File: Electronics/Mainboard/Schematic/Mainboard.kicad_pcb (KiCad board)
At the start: 4 copper layers, 45 x 140 mm, 84 parts, among them J1 CONN_01X02, J10 CONN_01X04, J11 M1, J12 M2, J13 M3, J14 M4, J2 CONN_01X02, J3 CONN_01X02, J4 CONN_01X02, J5 CONN_01X02, J6 CONN_02X05, J7 CONN_02X10, J8 CONN_01X02, J9 CONN_01X02, Q1 BUK7Y7R8-80EX, Q2 BUK7Y7R8-80EX, Q4 BUK7Y7R8-80EX, U1 LM2678-3.3V, U10 LTC2954, U2 LM2678-12V, U4 LM5121, U6 ACS781, U7 LSM6DS33, U8 STM32F031G6U6, U9 LTC2876, Y1 Resonator_Small

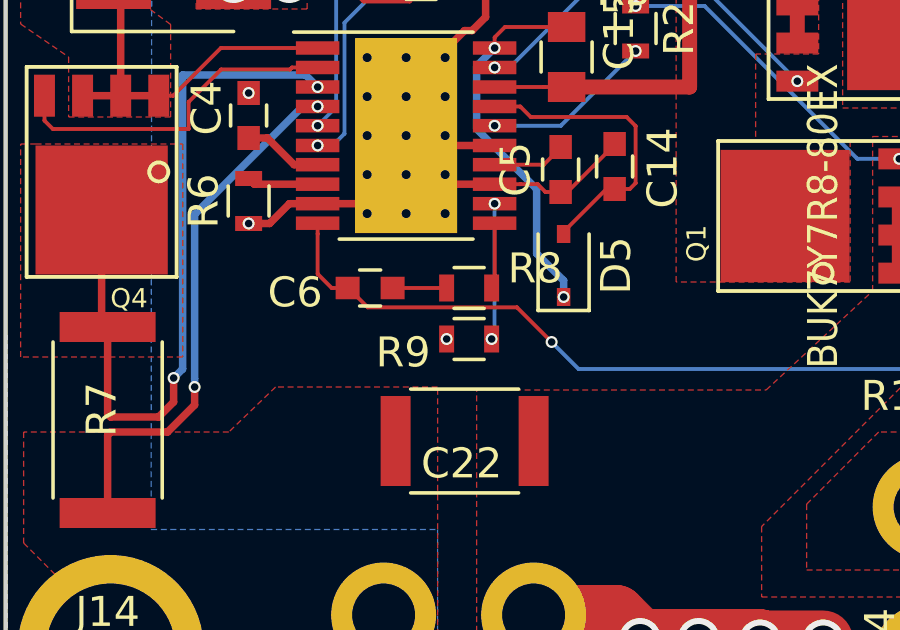
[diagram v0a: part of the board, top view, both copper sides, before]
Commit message: new mainboard
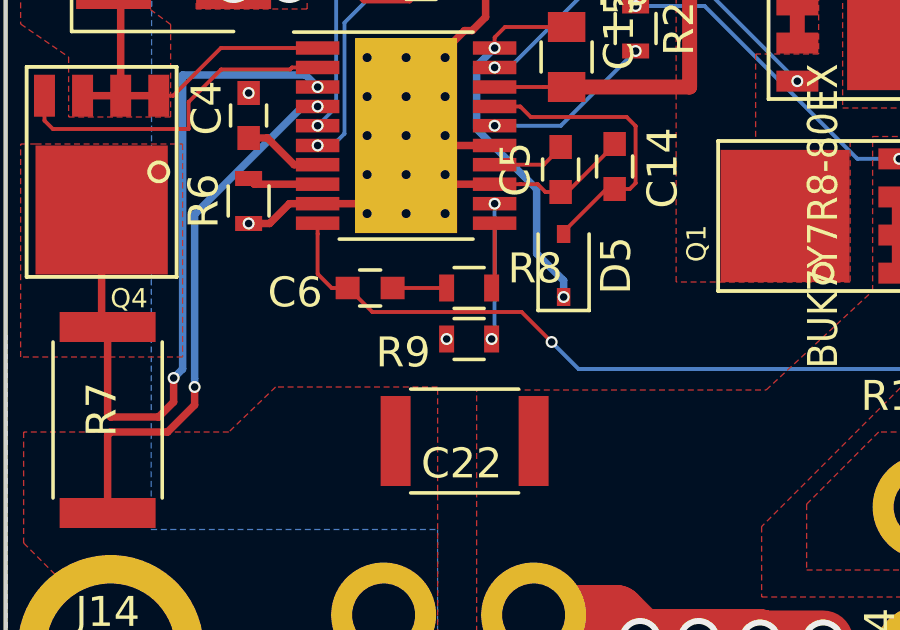
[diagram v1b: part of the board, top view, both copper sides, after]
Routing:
- net Earth: vias 56 -> 55
- net (no net): vias 0 -> 1
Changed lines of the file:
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@@
     (links 231)
     (no_connects 0)
-    (area 49.924999 29.924999 95.075001 170.075001)
+    (area 47.327142 29.924999 95.075001 170.763333)
     (thickness 1.6)
     (drawings 23)
@@
   )
   (setup
-    (last_trace_width 2)
+    (last_trace_width 0.13)
     (user_trace_width 0.13)
     (user_trace_width 0.25)
@@
     (visible_elements 7FFFEFFF)
     (pcbplotparams
-      (layerselection 0x010f0_80000001)
+      (layerselection 0x010f0_80000007)
       (usegerberextensions false)
       (excludeedgelayer true)
@@
   (gr_line (start 95 32) (end 95 168) (layer Edge.Cuts) (width 0.15))
   (gr_line (start 52 30) (end 93 30) (layer Edge.Cuts) (width 0.15))
+  (via (at 59.45 144.3) (size 1.4) (drill 1) (layers F.Cu B.Cu) (net 0))
   (via (at 54.9 99.6) (size 1.4) (drill 1) (layers F.Cu B.Cu) (net 1))
   (via (at 57.9 99.6) (size 1.4) (drill 1) (layers F.Cu B.Cu) (net 1))
-  (via (at 59.45 144.3) (size 1.4) (drill 1) (layers F.Cu B.Cu) (net 1))
   (segment (start 52.75 84.35) (end 55.35 84.35) (width 2) (layer F.Cu) (net 1))
   (via (at 55.35 84.35) (size 1.4) (drill 1) (layers F.Cu B.Cu) (net 1))
@@
   (segment (start 60.366596 148.45) (end 60.4 148.45) (width 0.25) (layer B.Cu) (net 4))
   (via (at 60.4 148.45) (size 0.4) (drill 0.25) (layers F.Cu B.Cu) (net 4))
+  (segment (start 61.4 154.5) (end 61.425 154.5) (width 0.13) (layer F.Cu) (net 5))
+  (segment (start 61.425 154.5) (end 62.225 155.3) (width 0.13) (layer F.Cu) (net 5))
+  (segment (start 67.2 155.3) (end 68.2 156.3) (width 0.13) (layer F.Cu) (net 5))
+  (segment (start 62.225 155.3) (end 67.2 155.3) (width 0.13) (layer F.Cu) (net 5))
   (segment (start 68.2 156.3) (end 69.1 157.2) (width 0.13) (layer B.Cu) (net 5))
   (segment (start 82.65 157.2) (end 83.45 158) (width 0.13) (layer B.Cu) (net 5))
@@
   (via (at 83.45 158) (size 0.4) (drill 0.25) (layers F.Cu B.Cu) (net 5))
   (segment (start 84.85 158) (end 83.45 158) (width 0.13) (layer F.Cu) (net 5))
-  (segment (start 61.4 154.5) (end 61.425 154.5) (width 0.13) (layer F.Cu) (net 5))
-  (segment (start 61.425 154.5) (end 62.070001 155.145001) (width 0.13) (layer F.Cu) (net 5))
-  (segment (start 62.070001 155.145001) (end 67.045001 155.145001) (width 0.13) (layer F.Cu) (net 5))
-  (segment (start 67.045001 155.145001) (end 68.2 156.3) (width 0.13) (layer F.Cu) (net 5))
   (via (at 68.2 156.3) (size 0.4) (drill 0.25) (layers F.Cu B.Cu) (net 5))
   (segment (start 61.4 154.5) (end 60.87 154.5) (width 0.13) (layer F.Cu) (net 5))
@@
     )
   )
-  (zone (net 1) (net_name Earth) (layer F.Mask) (hatch edge 0.508)
+  (zone (net 0) (net_name "") (layer F.Mask) (hatch edge 0.508)
     (connect_pads (clearance 0.508))
     (min_thickness 0.254)
@@
     )
   )
-  (zone (net 7) (net_name "Net-(C7-Pad2)") (layer F.Mask) (hatch edge 0.508)
+  (zone (net 0) (net_name "") (layer F.Mask) (hatch edge 0.508)
     (connect_pads (clearance 0.508))
     (min_thickness 0.254)
